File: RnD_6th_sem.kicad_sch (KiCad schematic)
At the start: 59 parts, among them IC1 2EDF7275KXUMA1, J1 HVDC, J10 MMCX-J-P-H-ST-TH1, J2 PWM, J3 HVDC, J4 Conn_01x06_Female, J5 5V, J6 5V, J7 GND, J8 GND, J9 MMCX-J-P-H-ST-TH1, Q1 IGLD60R190D1, Q2 IGLD60R190D1

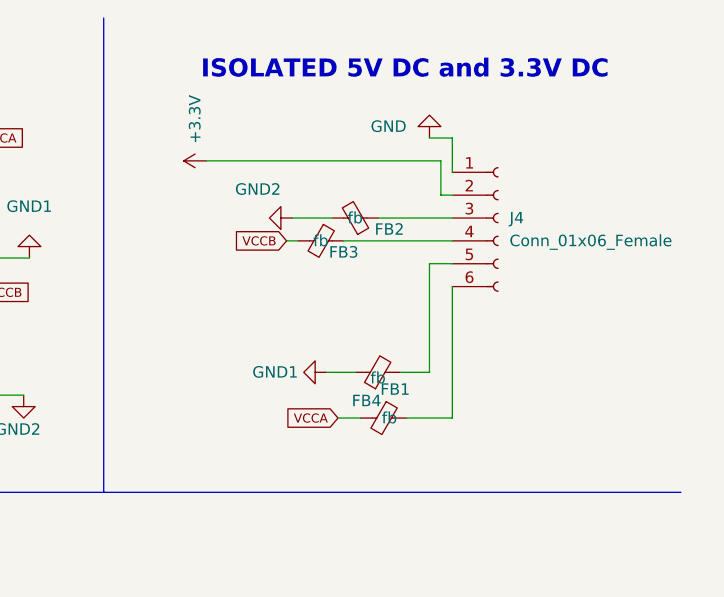
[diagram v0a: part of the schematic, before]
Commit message: Updated final design
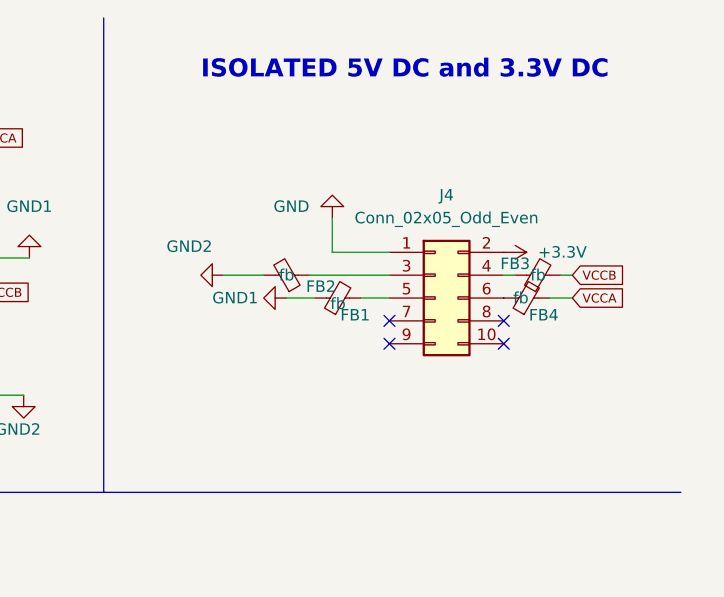
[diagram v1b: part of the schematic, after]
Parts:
- removed J4: Conn_01x06_Female, Connector_PinSocket_2.54mm:PinSocket_1x06_P2.54mm_Horizontal, symbol Connector:Conn_01x06_Female
- added J4: Conn_02x05_Odd_Even, 61201021621:SHDR10W64P254_2X5_2036X885X925P, symbol Connector_Generic:Conn_02x05_Odd_Even
- IC1: footprint 2EDF7275KXUMA1:2EDF7275KXUMA1 -> 2EDF7275K:TFLGA65P500X500X106-14_13N-V
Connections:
- net +3.3V: now also J4.2 (Pin_2)
- net GND: now also J4.1 (Pin_1)
- net at FB2.1: now also J4.3 (Pin_3)
- net at FB3.1: now also J4.4 (Pin_4)
- net at FB1.2: now also J4.5 (Pin_5)
- net at FB4.1: now also J4.6 (Pin_6)
- no-connect marks 0 -> 4
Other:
- moved on the sheet: FB1, FB2, FB3, FB4
